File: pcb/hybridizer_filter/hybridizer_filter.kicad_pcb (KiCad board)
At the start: 2 copper layers, 85.6 x 132.2 mm, 126 parts, among them P1 HEADER_02X07_SMD, P2 HEADER_02X05_SMD, P3 HEADER_02X05_SMD, U1 VA, U11 VA, U13 VA, U15 DRV103, U16 DRV103, U17 DRV103, U18 DRV103, U19 DRV103, U20 DRV103, U21 DRV103, U22 DRV103, U23 OA, U24 OA, U25 OA, U26 OA, U27 OA, U28 OA, U29 OA, U3 VA, U5 VA, U7 VA, U9 VA

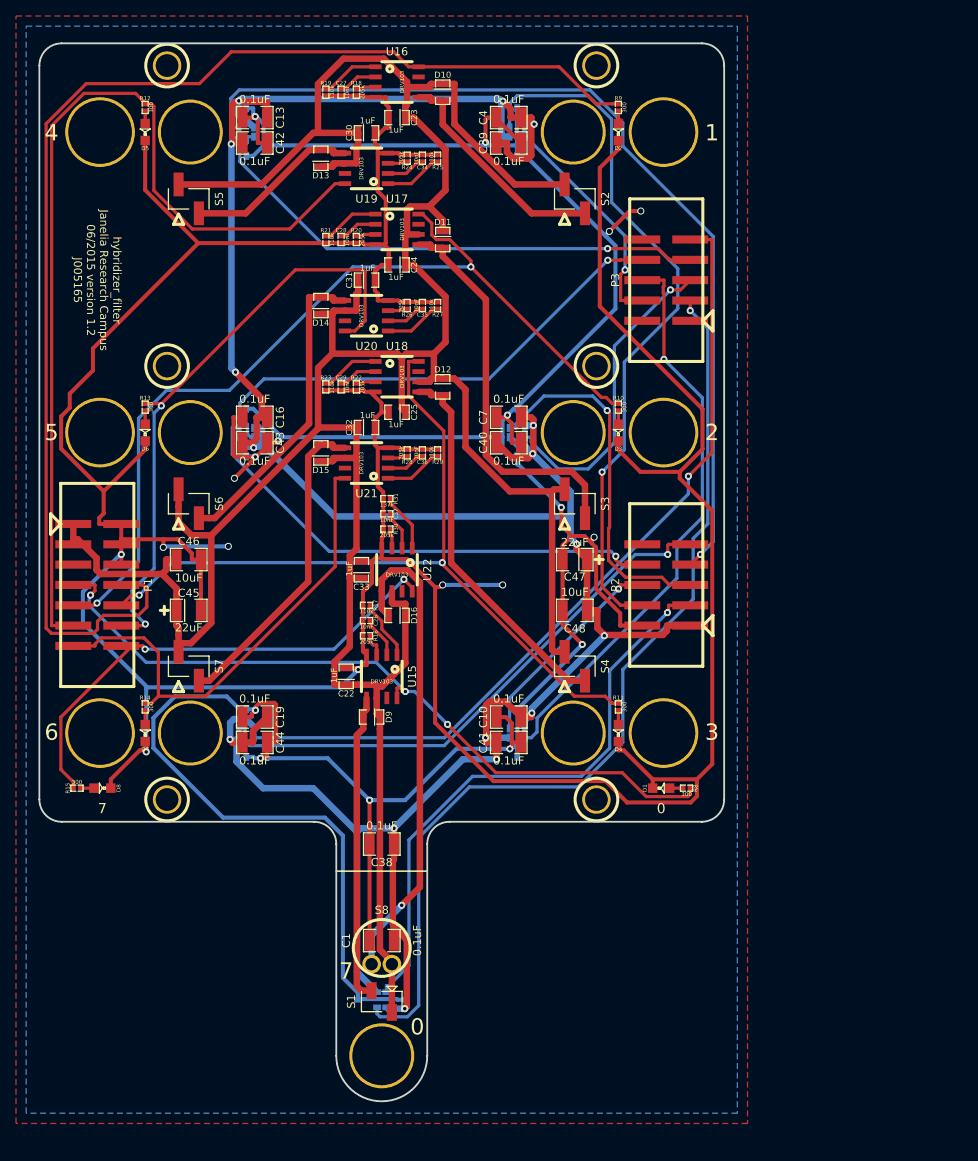
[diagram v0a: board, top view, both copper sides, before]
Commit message: Progress towards hybridizer_filter v1.0.
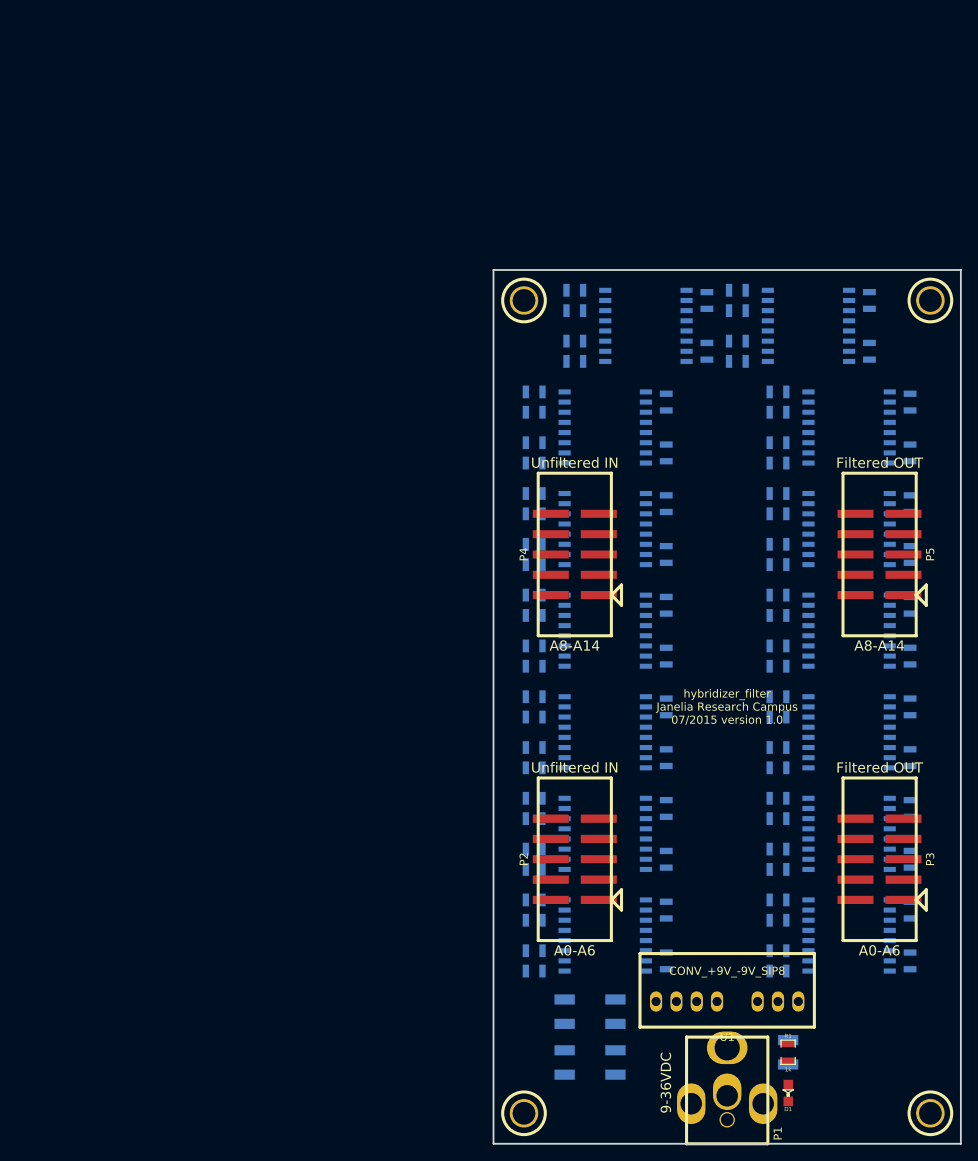
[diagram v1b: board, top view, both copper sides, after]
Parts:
- removed C34, C35, C36, C37: 10nF, hybridizer_filter:SM0402
- removed C38, C39, C40, C41, C42, C43, C44: 0.1uF, hybridizer_filter:SM1210
- removed C45, C47: 22uF, hybridizer_filter:SM1210_POL
- removed C46, C48: 10uF, hybridizer_filter:SM1210
- removed CLEARANCE_HOLE_1, CLEARANCE_HOLE_2, CLEARANCE_HOLE_3, CLEARANCE_HOLE_4, CLEARANCE_HOLE_5, CLEARANCE_HOLE_6: clearance_hole, hybridizer_filter:clearance_hole
- removed D10, D11, D12, D13, D14, D15, D16, D9: diode_schottky_20V_1A, hybridizer_filter:SM0805_POL
- removed D2, D3, D4, D5, D6, D7, D8: LED_0805, hybridizer_filter:LED0805
- removed MOUNTING_HOLE_1, MOUNTING_HOLE_2, MOUNTING_HOLE_3, MOUNTING_HOLE_4, MOUNTING_HOLE_5, MOUNTING_HOLE_6: mounting_hole, hybridizer_filter:mounting_hole
- removed REF**, VALVE_HOLE_1, VALVE_HOLE_2, VALVE_HOLE_3, VALVE_HOLE_4, VALVE_HOLE_5, VALVE_HOLE_6: valve_hole, hybridizer_filter:valve_hole
- removed S1: HEADER_01X02_SMD_N, hybridizer_filter:Header_2_Pin_SMD_N
- removed S2, S3, S4, S5, S6, S7: HEADER_01X02_SMD, hybridizer_filter:Header_2_Pin_SMD
- removed S8: LEE_VALVE_PLUG_IN, hybridizer_filter:LEE_VALVE_PLUG_IN
- removed U16, U17, U18, U19, U20, U21, U22: DRV103, hybridizer_filter:SOIC_8
- removed U23, U24, U25, U26, U27, U28, U29: OA, hybridizer_filter:SOT-23-3
- added C11: 0.1uF, hybridizer_filter:SM0805, B.Cu at (112.6, 90.6)
- added C12: 0.1uF, hybridizer_filter:SM0805, B.Cu at (112.6, 100.7)
- added C14: 0.1uF, hybridizer_filter:SM0805, B.Cu at (112.6, 113.4)
- added C15: 0.1uF, hybridizer_filter:SM0805, B.Cu at (112.6, 116.0)
- added C17: 0.1uF, hybridizer_filter:SM0805, B.Cu at (112.6, 128.7)
- added C18: 0.1uF, hybridizer_filter:SM0805, B.Cu at (112.6, 138.8)
- added C2: 22uF, hybridizer_filter:SM1210_POL, B.Cu at (116.5, 152.8)
- added C20: 0.1uF, hybridizer_filter:SM0805, B.Cu at (138.0, 62.6)
- added C21: 0.1uF, hybridizer_filter:SM0805, B.Cu at (138.0, 65.2)
- added C3: 10uF, hybridizer_filter:SM1210, B.Cu at (122.8, 152.8)
- added C5: 10uF, hybridizer_filter:SM1210, B.Cu at (122.8, 146.4)
- added C6: 0.1uF, hybridizer_filter:SM0805, B.Cu at (117.7, 62.6)
- added C8: 0.1uF, hybridizer_filter:SM0805, B.Cu at (112.6, 75.3)
- added C9: 0.1uF, hybridizer_filter:SM0805, B.Cu at (112.6, 77.9)
- added MH1: mounting_hole, hybridizer_filter:mounting_hole, F.Cu at (111.4, 57.5)
- added MH2: mounting_hole, hybridizer_filter:mounting_hole, F.Cu at (162.2, 57.5)
- added MH3: mounting_hole, hybridizer_filter:mounting_hole, F.Cu at (111.4, 159.1)
- added MH4: mounting_hole, hybridizer_filter:mounting_hole, F.Cu at (162.2, 159.1)
- added P4: HEADER_02X05_SMD, hybridizer_filter:HEADER_02x05_SMD, F.Cu at (117.7, 89.3)
- added P5: HEADER_02X05_SMD, hybridizer_filter:HEADER_02x05_SMD, F.Cu at (155.8, 89.3)
- added R1: 1k, hybridizer_filter:SM0805, F.Cu at (144.4, 151.5)
- added R2: 3.16M, hybridizer_filter:SM0805, B.Cu at (117.7, 56.3)
- added R3: 3.16M, hybridizer_filter:SM0805, B.Cu at (134.2, 63.9)
- added R32: 49.9k, hybridizer_filter:SM0805, B.Cu at (138.0, 58.8)
- added R33: 42.2k, hybridizer_filter:SM0805, B.Cu at (154.6, 57.5)
- added R34: 3.16M, hybridizer_filter:SM0805, B.Cu at (143.1, 69.0)
- added R35: 3.16M, hybridizer_filter:SM0805, B.Cu at (159.6, 76.6)
- added R36: 49.9k, hybridizer_filter:SM0805, B.Cu at (143.1, 71.5)
- added R37: 42.2k, hybridizer_filter:SM0805, B.Cu at (159.6, 70.2)
- added R38: 3.16M, hybridizer_filter:SM0805, B.Cu at (143.1, 81.7)
- added R39: 3.16M, hybridizer_filter:SM0805, B.Cu at (159.6, 89.3)
- added R4: 49.9k, hybridizer_filter:SM0805, B.Cu at (117.7, 58.8)
- added R40: 49.9k, hybridizer_filter:SM0805, B.Cu at (143.1, 84.2)
- added R41: 42.2k, hybridizer_filter:SM0805, B.Cu at (159.6, 82.9)
- added R42: 3.16M, hybridizer_filter:SM0805, B.Cu at (143.1, 94.4)
- added R43: 3.16M, hybridizer_filter:SM0805, B.Cu at (159.6, 102.0)
- added R44: 49.9k, hybridizer_filter:SM0805, B.Cu at (143.1, 96.9)
- added R45: 42.2k, hybridizer_filter:SM0805, B.Cu at (159.6, 95.6)
- added R46: 3.16M, hybridizer_filter:SM0805, B.Cu at (143.1, 107.1)
- added R47: 3.16M, hybridizer_filter:SM0805, B.Cu at (159.6, 114.7)
- added R48: 49.9k, hybridizer_filter:SM0805, B.Cu at (143.1, 109.6)
- added R49: 42.2k, hybridizer_filter:SM0805, B.Cu at (159.6, 108.3)
- added R5: 42.2k, hybridizer_filter:SM0805, B.Cu at (134.2, 57.5)
- added R50: 3.16M, hybridizer_filter:SM0805, B.Cu at (143.1, 119.8)
- added R51: 3.16M, hybridizer_filter:SM0805, B.Cu at (159.6, 127.4)
- added R52: 49.9k, hybridizer_filter:SM0805, B.Cu at (143.1, 122.3)
- added R53: 42.2k, hybridizer_filter:SM0805, B.Cu at (159.6, 121.0)
- added R54: 3.16M, hybridizer_filter:SM0805, B.Cu at (143.1, 132.5)
- added R55: 3.16M, hybridizer_filter:SM0805, B.Cu at (159.6, 140.1)
- added R56: 49.9k, hybridizer_filter:SM0805, B.Cu at (143.1, 135.0)
- added R57: 42.2k, hybridizer_filter:SM0805, B.Cu at (159.6, 133.7)
- added R6: 3.16M, hybridizer_filter:SM0805, B.Cu at (112.6, 69.0)
- added R7: 3.16M, hybridizer_filter:SM0805, B.Cu at (129.2, 76.6)
- added U10: UAF42, hybridizer_filter:SOIC_16, B.Cu at (152.0, 72.8)
- added U12: UAF42, hybridizer_filter:SOIC_16, B.Cu at (152.0, 98.2)
- added U14: UAF42, hybridizer_filter:SOIC_16, B.Cu at (152.0, 123.6)
- added U2: UAF42, hybridizer_filter:SOIC_16, B.Cu at (126.6, 60.1)
- added U4: UAF42, hybridizer_filter:SOIC_16, B.Cu at (121.5, 85.5)
- added U6: UAF42, hybridizer_filter:SOIC_16, B.Cu at (121.5, 110.9)
- added U8: UAF42, hybridizer_filter:SOIC_16, B.Cu at (121.5, 136.3)
- C1: value 0.1uF -> 10uF; moved to B.Cu
- C10, C13, C16, C19, C7: footprint hybridizer_filter:SM1210 -> hybridizer_filter:SM0805; moved to B.Cu
- C22, C23, C24, C25, C30, C31, C32, C33: value 1uF -> 0.1uF; footprint hybridizer_filter:SM0805_POL -> hybridizer_filter:SM0805; moved to B.Cu
- C26, C27, C28, C29: value 10nF -> 0.1uF; footprint hybridizer_filter:SM0402 -> hybridizer_filter:SM0805; moved to B.Cu
- C4: value 0.1uF -> 22uF; footprint hybridizer_filter:SM1210 -> hybridizer_filter:SM1210_POL; moved to B.Cu
- P1: value HEADER_02X07_SMD -> PWR_JACK_2.1x5.5; footprint hybridizer_filter:HEADER_02x07_SMD -> hybridizer_filter:DCJACK_2PIN_HIGHCURRENT
- R10, R11, R14, R15: value 300 -> 3.16M; footprint hybridizer_filter:SM0402 -> hybridizer_filter:SM0805; moved to B.Cu
- R12, R8: value 300 -> 49.9k; footprint hybridizer_filter:SM0402 -> hybridizer_filter:SM0805; moved to B.Cu
- R13, R9: value 300 -> 42.2k; footprint hybridizer_filter:SM0402 -> hybridizer_filter:SM0805; moved to B.Cu
- R16, R20, R24, R28: value 205k -> 49.9k; footprint hybridizer_filter:SM0402 -> hybridizer_filter:SM0805; moved to B.Cu
- R17, R21, R25, R29: value 110k -> 42.2k; footprint hybridizer_filter:SM0402 -> hybridizer_filter:SM0805; moved to B.Cu
- R18, R22, R26, R30: value 205k -> 3.16M; footprint hybridizer_filter:SM0402 -> hybridizer_filter:SM0805; moved to B.Cu
- R19, R23, R27: value 110k -> 3.16M; footprint hybridizer_filter:SM0402 -> hybridizer_filter:SM0805; moved to B.Cu
- R31: value 137k -> 3.16M; footprint hybridizer_filter:SM0402 -> hybridizer_filter:SM0805; moved to B.Cu
- U1: value VA -> CONV_+9V_-9V_SIP8; footprint hybridizer_filter:SOT-23-3 -> hybridizer_filter:SIP8_RECOM; moved to F.Cu
- U11, U13, U3, U5, U7, U9: value VA -> UAF42; footprint hybridizer_filter:SOT-23-3 -> hybridizer_filter:SOIC_16
- U15: value DRV103 -> UAF42; footprint hybridizer_filter:SOIC_8 -> hybridizer_filter:SOIC_16; moved to B.Cu
- moved C4 112.0 mm to (116.5, 146.4), turned to 90 degrees
- moved P1 105.3 mm to (136.8, 163.0), turned to 180 degrees
- moved C30 103.3 mm to (143.1, 126.1), turned to 180 degrees
- moved R19 93.4 mm to (129.2, 114.7)
- moved C27 90.2 mm to (143.1, 103.3), turned to 0 degrees
- moved C31 89.8 mm to (143.1, 128.7)
- moved R27 86.8 mm to (129.2, 140.1), turned to 270 degrees
- moved R25 86.2 mm to (129.2, 121.0)
- moved R24 84.1 mm to (112.6, 122.3), turned to 180 degrees
- moved C28 83.8 mm to (143.1, 113.4), turned to 180 degrees
- moved C32 83.2 mm to (143.1, 138.8), turned to 180 degrees
- moved R18 78.8 mm to (112.6, 107.1), turned to 0 degrees
- moved P3 77.1 mm to (155.8, 127.4)
- moved C13 77.0 mm to (112.6, 103.3), turned to 0 degrees
- moved U11 76.5 mm to (152.0, 85.5)
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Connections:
- C1 pad 1: +5V -> VAA
- C1 pad 2: GNDA -> GND
- C10 pad 1: +5V -> VDD
- C13 pad 1: +5V -> GNDA
- C13 pad 2: GNDA -> VEE
- C16 pad 1: +5V -> VDD
- C19 pad 1: +5V -> GNDA
- C19 pad 2: GNDA -> VEE
- C22 pad 1: VAA -> VDD
- C22 pad 2: GND -> GNDA
- C23 pad 1: VAA -> GNDA
- C23 pad 2: GND -> VEE
- C24 pad 1: VAA -> VDD
- C24 pad 2: GND -> GNDA
- C25 pad 1: VAA -> GNDA
- C25 pad 2: GND -> VEE
- C26 pad 1: Net-(C26-Pad1) -> VDD
- C26 pad 2: GND -> GNDA
- C27 pad 1: Net-(C27-Pad1) -> GNDA
- C27 pad 2: GND -> VEE
- C28 pad 1: Net-(C28-Pad1) -> VDD
- C28 pad 2: GND -> GNDA
- C29 pad 1: Net-(C29-Pad1) -> GNDA
- C29 pad 2: GND -> VEE
- C30 pad 1: VAA -> VDD
- C30 pad 2: GND -> GNDA
- C31 pad 1: VAA -> GNDA
- C31 pad 2: GND -> VEE
- C32 pad 1: VAA -> VDD
- C32 pad 2: GND -> GNDA
- C33 pad 1: VAA -> GNDA
- C33 pad 2: GND -> VEE
- C4 pad 1: +5V -> GNDA
- C4 pad 2: GNDA -> VEE
- C7 pad 1: +5V -> GNDA
- C7 pad 2: GNDA -> VEE
- P2 pad 1: +5V -> /Va
- P3 pad 1: Net-(P3-Pad1) -> /Va
- P3 pad 2: Net-(P3-Pad2) -> GNDA
- P3 pad 3: /A8 -> /A0_F
- P3 pad 4: /A9 -> /A1_F
- P3 pad 5: /A10 -> /A2_F
- P3 pad 6: /A11 -> /A3_F
- P3 pad 7: /A12 -> /A4_F
- P3 pad 8: /A13 -> /A5_F
- P3 pad 9: /A14 -> /A6_F
- R10 pad 1: /IO2 -> Net-(R10-Pad1)
- R11 pad 1: /IO3 -> Net-(R11-Pad1)
- R12 pad 1: /IO4 -> Net-(R12-Pad1)
- R12 pad 2: Net-(D5-Pad1) -> /A2
- R13 pad 1: /IO5 -> Net-(R13-Pad1)
- R13 pad 2: Net-(D6-Pad1) -> GNDA
- R14 pad 1: /IO6 -> Net-(R14-Pad1)
- R14 pad 2: Net-(D7-Pad1) -> Net-(R14-Pad2)
- R15 pad 1: /IO7 -> Net-(R15-Pad1)
- R15 pad 2: Net-(D8-Pad1) -> Net-(R15-Pad2)
- R16 pad 2: GND -> /A3
- R17 pad 2: GND -> GNDA
- R18 pad 2: GND -> Net-(R18-Pad2)
- R19 pad 2: GND -> Net-(R19-Pad2)
- R20 pad 2: GND -> /A4
- R21 pad 2: GND -> GNDA
- R22 pad 2: GND -> Net-(R22-Pad2)
- R23 pad 2: GND -> Net-(R23-Pad2)
- R24 pad 2: GND -> /A5
- R25 pad 2: GND -> GNDA
- R26 pad 2: GND -> Net-(R26-Pad2)
- R27 pad 2: GND -> Net-(R27-Pad2)
- R28 pad 2: GND -> /A6
- R29 pad 2: GND -> GNDA
- R30 pad 2: GND -> Net-(R30-Pad2)
- R31 pad 2: GND -> Net-(R31-Pad2)
- R8 pad 1: /IO0 -> Net-(R8-Pad1)
- R8 pad 2: Net-(D1-Pad1) -> /A1
- R9 pad 1: /IO1 -> Net-(R9-Pad1)
- R9 pad 2: Net-(D2-Pad1) -> GNDA
- U1 pad 1: +5V -> GND
- U1 pad 2: /A0 -> VAA
- U1 pad 3: GNDA -> (no net)
- U11 pad 1: +5V -> /A10_LP
- U11 pad 2: /A5 -> GNDA
- U11 pad 3: GNDA -> Net-(U11-Pad3)
- U13 pad 1: +5V -> /A12_LP
- U13 pad 2: /A6 -> GNDA
- U13 pad 3: GNDA -> Net-(U13-Pad3)
- U15 pad 1: Net-(R17-Pad1) -> /A14_LP
- U15 pad 2: Net-(C26-Pad1) -> GNDA
- U15 pad 3: Net-(R16-Pad1) -> Net-(U15-Pad3)
- U15 pad 4: GND -> Net-(R57-Pad1)
- U15 pad 5: /SH0 -> /A14_LP
- U15 pad 6: VAA -> /A14_F
- U15 pad 7: Net-(U15-Pad7) -> /A14_F
- U15 pad 8: /IO0 -> Net-(R55-Pad2)
- U3 pad 1: +5V -> /A1_LP
- U3 pad 2: /A1 -> GNDA
- U3 pad 3: GNDA -> Net-(U3-Pad3)
- U5 pad 1: +5V -> /A3_LP
- U5 pad 2: /A2 -> GNDA
- U5 pad 3: GNDA -> Net-(U5-Pad3)
- U7 pad 1: +5V -> /A5_LP
- U7 pad 2: /A3 -> GNDA
- U7 pad 3: GNDA -> Net-(U7-Pad3)
- U9 pad 1: +5V -> /A8_LP
- U9 pad 2: /A4 -> GNDA
- U9 pad 3: GNDA -> Net-(U9-Pad3)
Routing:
- net GND: track 487.3 -> 0.00 mm, vias 7 -> 0
- net VAA: track 408.7 -> 0.00 mm
- net GNDA: track 390.6 -> 0.00 mm, vias 15 -> 0
- net +5V: track 360.5 -> 0.00 mm, vias 16 -> 0
- net /IO1: track 161.5 -> 0.00 mm
- net /IO4: track 119.2 -> 0.00 mm
- net /A8: track 118.7 -> 0.00 mm, vias 1 -> 0
- net /A4: track 116.7 -> 0.00 mm, vias 1 -> 0
- net /IO2: track 113.8 -> 0.00 mm, vias 2 -> 0
- net /A14: track 102.6 -> 0.00 mm, vias 1 -> 0
- net /IO3: track 100.0 -> 0.00 mm, vias 2 -> 0
- net /IO0: track 93.9 -> 0.00 mm, vias 3 -> 0
- net /A1: track 89.2 -> 0.00 mm, vias 1 -> 0
- net /IO5: track 76.5 -> 0.00 mm, vias 2 -> 0
- net /A0: track 73.8 -> 0.00 mm, vias 1 -> 0
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- removed copper zone on F.Cu, net GND
- removed copper zone on B.Cu, net GNDA
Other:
- board size 85.6 x 132.2 mm -> 58.4 x 109.2 mm
- board text added: "9-36VDC"
- board text added: "A0-A6"
- board text added: "A8-A14"
- board text added: "Filtered OUT"
- board text added: "Unfiltered IN"
- board text added: "hybridizer_filter Janelia Research Campus 07/2015 version 1.0"
- board text removed: "0"
- board text removed: "1"
- board text removed: "2"
- board text removed: "3"
- board text removed: "4"
- board text removed: "5"
- board text removed: "6"
- board text removed: "7"
- board text removed: "hybridizer_filter Janelia Research Campus 06/2015 version 1.2 J005165"
